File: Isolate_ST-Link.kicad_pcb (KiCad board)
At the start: 2 copper layers, 46.5 x 50 mm, 66 parts, among them J1 USB_OTG, J2 CONN_01X06, J3 CONN_01X04, J4 CONN_01X02, J5 CONN_01X02, J6 GS2, Q1 BSS138, U1 MAU10x, U2 ADuM4160, U3 APE8865NR-33-HF-3, U4 STM32F103CBTx, Y1 Crystal

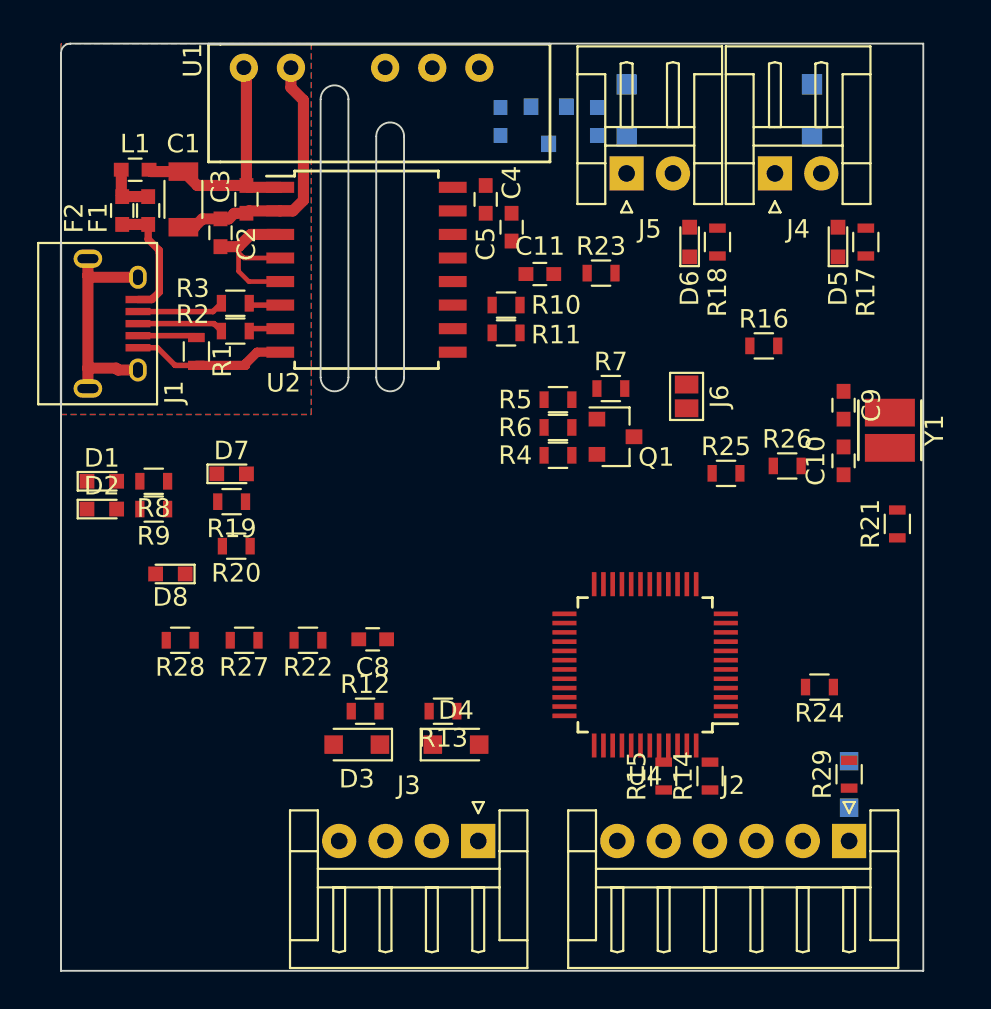
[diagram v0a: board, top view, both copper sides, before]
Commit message: AW進捗
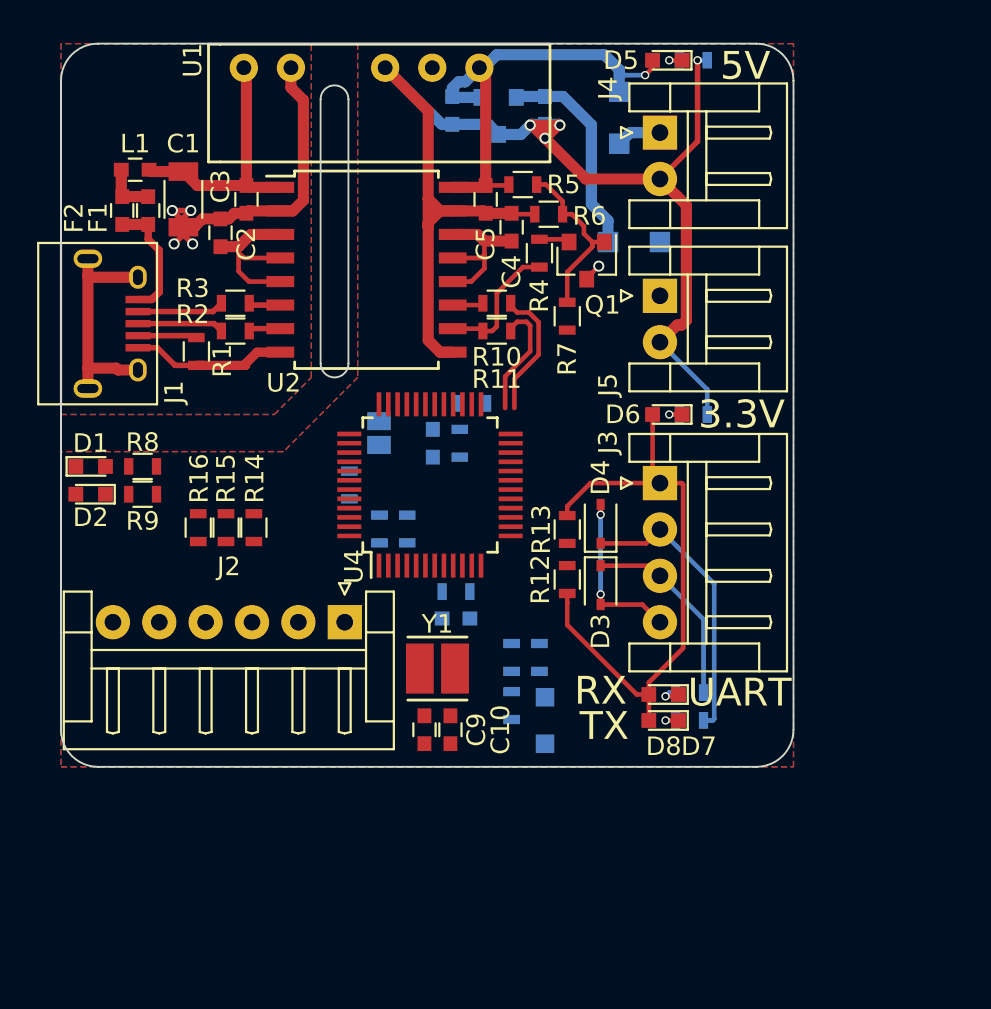
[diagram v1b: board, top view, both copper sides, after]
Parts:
- C11, C8, J6, R17, R18, R19, R20, R21, R22, R23, R24, R25, R26, R27, R28, R29: moved to B.Cu
- D3, D4: footprint Diodes_SMD:D_SOD-323_HandSoldering -> Diodes_SMD:D_SOD-323
- moved R16 32.0 mm to (160.9, 76.1), turned to 90 degrees
- moved J2 29.6 mm to (168.8, 81.2)
- moved C9 28.6 mm to (173.1, 87.0), turned to 90 degrees
- moved R14 28.0 mm to (163.9, 76.1)
- moved D8 27.7 mm to (186.0, 86.5)
- moved R24 27.6 mm to (169.1, 73.8), turned to 90 degrees
- moved Y1 27.6 mm to (173.8, 83.7), turned to 0 degrees
- moved R15 27.1 mm to (162.4, 76.1)
- moved R19 26.8 mm to (187.4, 85.0)
- moved R20 26.2 mm to (187.4, 86.5)
- moved D7 26.2 mm to (186.0, 85.1), turned to 180 degrees
- moved C10 25.7 mm to (174.5, 87.0)
- moved R21 24.1 mm to (174.8, 79.5), turned to 180 degrees
- moved J3 21.6 mm to (185.8, 73.7), turned to 270 degrees
- moved R28 19.4 mm to (179.3, 83.1), turned to 90 degrees
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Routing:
- net GND: track 0.00 -> 79.1 mm, vias 0 -> 6
- net +3V3: track 0.00 -> 44.7 mm, vias 0 -> 1
- net +5V: track 0.00 -> 25.6 mm, vias 0 -> 1
- net /MCU/UART_TX: track 0.00 -> 15.6 mm
- net /MCU/UART_RX: track 0.00 -> 10.7 mm
- net Net-(Q1-Pad1): track 0.00 -> 9.39 mm
- net Net-(C4-Pad2): track 0.00 -> 8.59 mm
- net Net-(R11-Pad2): track 0.00 -> 7.20 mm
- net /MCU/USB_DM: track 0.00 -> 7.18 mm
- net /MCU/USB_DP: track 0.00 -> 6.44 mm
- net GNDPWR: track 35.4 -> 40.4 mm, vias 0 -> 4
- net Net-(D9-Pad1): track 0.00 -> 2.45 mm
- net Net-(R10-Pad1): track 0.00 -> 1.67 mm
- net Net-(Q1-Pad2): track 0.00 -> 1.66 mm
- net Net-(D7-Pad1): track 0.00 -> 1.37 mm, vias 0 -> 1
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- added copper zone on B.Cu, net GND
- added copper zone on F.Cu, net GND
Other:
- board size 46.5 x 50 mm -> 39.5 x 39 mm
- board text added: "3.3V"
- board text added: "5V"
- board text added: "RX"
- board text added: "TX"
- board text added: "UART"
